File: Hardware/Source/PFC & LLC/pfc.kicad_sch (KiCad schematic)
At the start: 56 parts, among them J1 HB9500M-9.5-3P, K1 Relay 12VDC 10A, Q1 MMBT2222A, Q2 IPP60R125CP, Q3 MMBT2222A, U2 PC817X2NIPW, U3 SN74LVC1G14DBVR, U4 UCC28180D

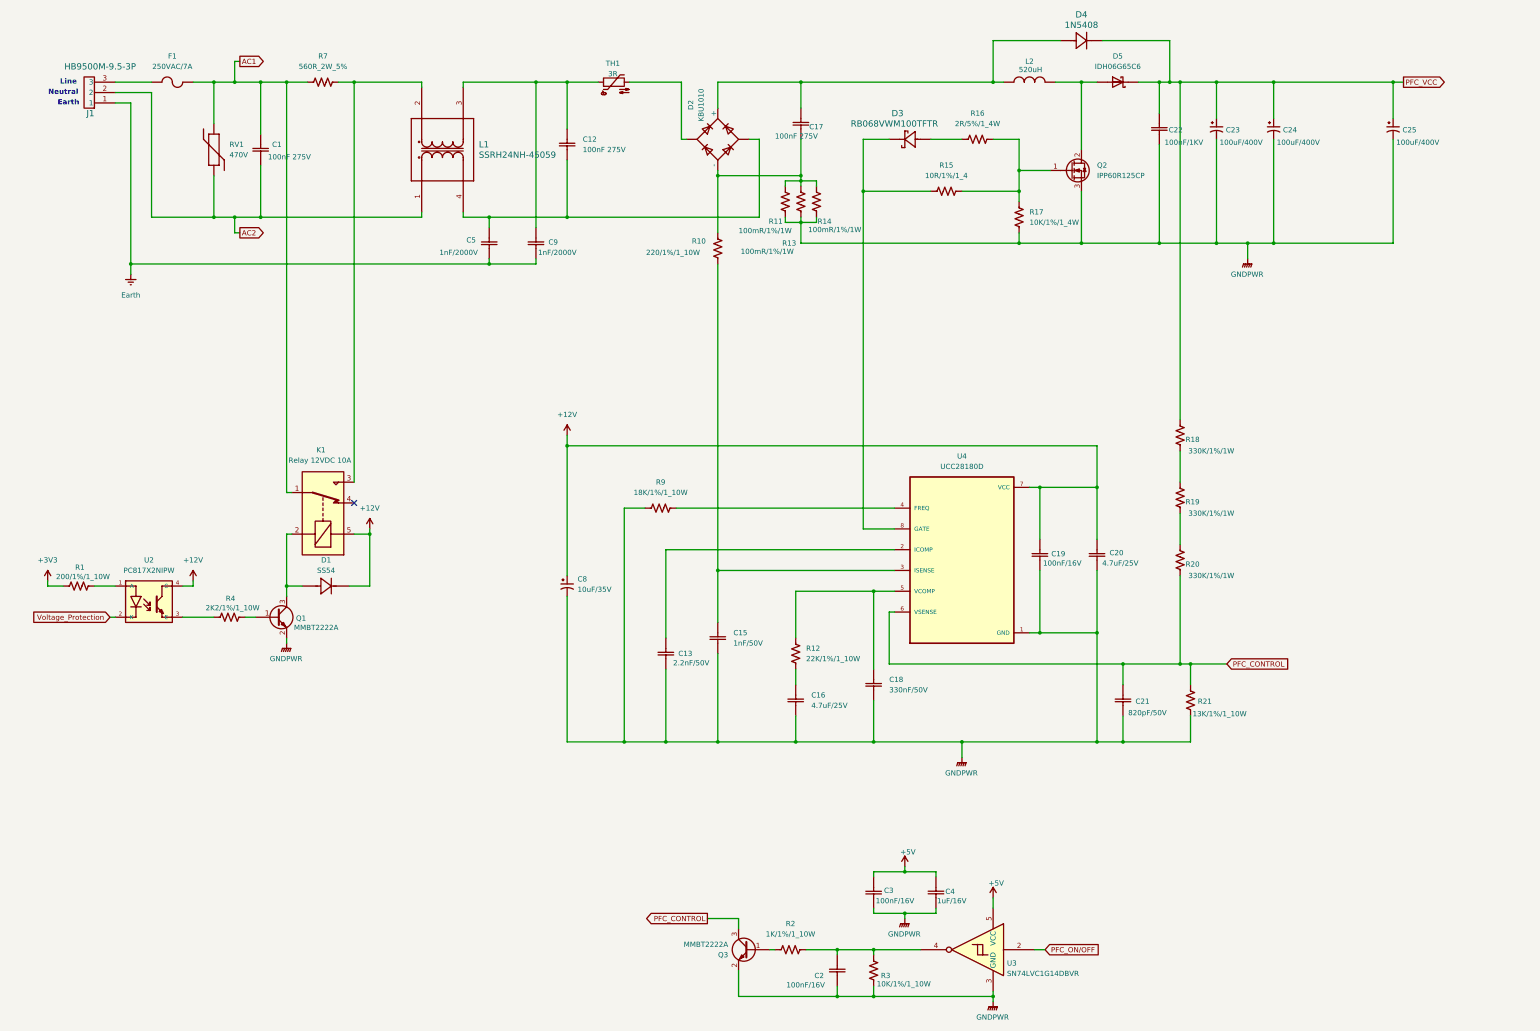
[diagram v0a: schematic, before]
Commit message: update FEEDBACK, AC
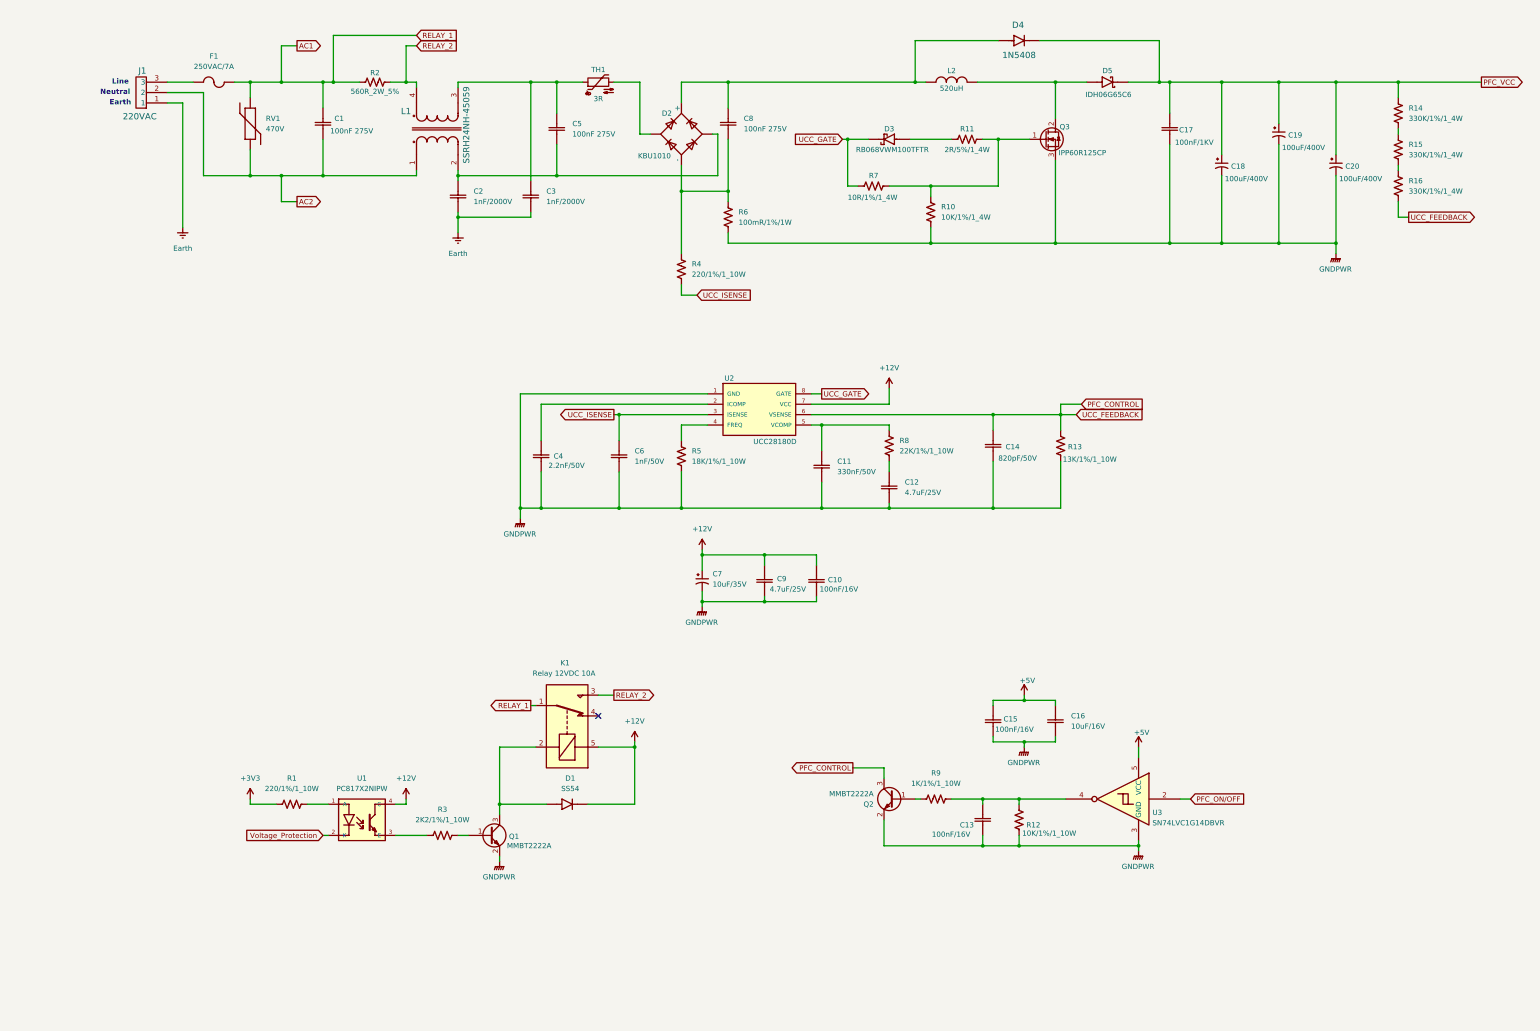
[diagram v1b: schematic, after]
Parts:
- removed C13: 2.2nF/50V, charge_battery_footprint_lib:Ceramic_Cap_0805, symbol charge_battery_sym_lib:Ceramic_Cap_SMD_2.2nF_50V
- removed C15: 1nF/50V, charge_battery_footprint_lib:Ceramic_Cap_0603, symbol charge_battery_sym_lib:Ceramic_Cap_SMD_1nF_50V
- removed C16, C20: 4.7uF/25V, charge_battery_footprint_lib:Ceramic_Cap_0603, symbol charge_battery_sym_lib:Ceramic_Cap_SMD_4.7uF_25V
- removed C17: 100nF 275V, charge_battery_footprint_lib:Candy_Cap_hole_100nF_275V, symbol charge_battery_sym_lib:Candy_Cap_hole_100nF_275V
- removed C18: 330nF/50V, charge_battery_footprint_lib:Ceramic_Cap_0603, symbol charge_battery_sym_lib:Ceramic_Cap_SMD_330nF_50V
- removed C19: 100nF/16V, charge_battery_footprint_lib:Ceramic_Cap_0603, symbol charge_battery_sym_lib:Ceramic_Cap_SMD_100nF_16V
- removed C21: 820pF/50V, charge_battery_footprint_lib:Ceramic_Cap_0805, symbol charge_battery_sym_lib:Ceramic_Cap_SMD_820pF_50V
- removed C4: 1uF/16V, charge_battery_footprint_lib:Ceramic_Cap_0603, symbol charge_battery_sym_lib:Ceramic_Cap_SMD_1uF_16V
- removed C5, C9: 1nF/2000V, charge_battery_footprint_lib:Ceramic_Cap_Hole_5mm, symbol charge_battery_sym_lib:Ceramic_Cap_Hole_1nF_2000V
- removed C8: 10uF/35V, charge_battery_footprint_lib:Tan_Cap_C, symbol charge_battery_sym_lib:Cap_Tantalum_10uF_35V
- removed L1: SSRH24NH-45059, charge_battery_footprint_lib:TPCM-1.7-5, symbol charge_battery_sym_lib:TPCM-1.7-5
- removed R1: 200/1%/1_10W, charge_battery_footprint_lib:Res_0603, symbol charge_battery_sym_lib:Res_200R_0603_1%
- removed R10: 220/1%/1_10W, charge_battery_footprint_lib:Res_0603, symbol charge_battery_sym_lib:Res_220R_0603_1%
- removed R11, R13, R14: 100mR/1%/1W, charge_battery_footprint_lib:Res_1206, symbol charge_battery_sym_lib:Res_100mR_1206_1%
- removed R12: 22K/1%/1_10W, charge_battery_footprint_lib:Res_0603, symbol charge_battery_sym_lib:Res_22K_0603_1%
- removed R18, R19, R20: 330K/1%/1W, charge_battery_footprint_lib:Res_1206, symbol charge_battery_sym_lib:Res_330K_1206_1%
- removed R21: 13K/1%/1_10W, charge_battery_footprint_lib:Res_0603, symbol charge_battery_sym_lib:Res_13K_0603_1%
- removed R4: 2K2/1%/1_10W, charge_battery_footprint_lib:Res_0603, symbol charge_battery_sym_lib:Res_2K2_0603_1%
- removed R9: 18K/1%/1_10W, charge_battery_footprint_lib:Res_0603, symbol charge_battery_sym_lib:Res_18K_0603_1%
- removed U4: UCC28180D, charge_battery_footprint_lib:SOIC-8, symbol charge_battery_sym_lib:UCC28180D
- added C10: 100nF/16V, charge_battery_footprint_lib:Ceramic_Cap_0603, symbol charge_battery_sym_lib:Ceramic_Cap_SMD_100nF_16V
- added C11: 330nF/50V, charge_battery_footprint_lib:Ceramic_Cap_0603, symbol charge_battery_sym_lib:Ceramic_Cap_SMD_330nF_50V
- added C12, C9: 4.7uF/25V, charge_battery_footprint_lib:Ceramic_Cap_0603, symbol charge_battery_sym_lib:Ceramic_Cap_SMD_4.7uF_25V
- added C14: 820pF/50V, charge_battery_footprint_lib:Ceramic_Cap_0805, symbol charge_battery_sym_lib:Ceramic_Cap_SMD_820pF_50V
- added C16: 10uF/16V, charge_battery_footprint_lib:Ceramic_Cap_0603, symbol charge_battery_sym_lib:Ceramic_Cap_SMD_10uF_16V
- added C2, C3: 1nF/2000V, charge_battery_footprint_lib:Ceramic_Cap_Hole_5mm, symbol charge_battery_sym_lib:Ceramic_Cap_Hole_1nF_2000V
- added C4: 2.2nF/50V, charge_battery_footprint_lib:Ceramic_Cap_0805, symbol charge_battery_sym_lib:Ceramic_Cap_SMD_2.2nF_50V
- added C6: 1nF/50V, charge_battery_footprint_lib:Ceramic_Cap_0603, symbol charge_battery_sym_lib:Ceramic_Cap_SMD_1nF_50V
- added C7: 10uF/35V, charge_battery_footprint_lib:Tan_Cap_C, symbol charge_battery_sym_lib:Cap_Tantalum_10uF_35V
- added C8: 100nF 275V, charge_battery_footprint_lib:Candy_Cap_hole_100nF_275V, symbol charge_battery_sym_lib:Candy_Cap_hole_100nF_275VAC
- added L1: SSRH24NH-45059, charge_battery_footprint_lib:SSRH24NH-45059, symbol charge_battery_sym_lib:SSRH24NH-45059
- added R1, R4: 220/1%/1_10W, charge_battery_footprint_lib:Res_0603, symbol charge_battery_sym_lib:Res_220R_0603_1%
- added R13: 13K/1%/1_10W, charge_battery_footprint_lib:Res_0603, symbol charge_battery_sym_lib:Res_13K_0603_1%
- added R14, R15, R16: 330K/1%/1_4W, charge_battery_footprint_lib:Res_1206, symbol charge_battery_sym_lib:Res_330K_1206_1%
- added R3: 2K2/1%/1_10W, charge_battery_footprint_lib:Res_0603, symbol charge_battery_sym_lib:Res_2K2_0603_1%
- added R5: 18K/1%/1_10W, charge_battery_footprint_lib:Res_0603, symbol charge_battery_sym_lib:Res_18K_0603_1%
- added R6: 100mR/1%/1W, charge_battery_footprint_lib:Res_1206, symbol charge_battery_sym_lib:Res_100mR_1206_1%
- added R8: 22K/1%/1_10W, charge_battery_footprint_lib:Res_0603, symbol charge_battery_sym_lib:Res_22K_0603_1%
- added U2: UCC28180D, charge_battery_footprint_lib:SOIC-8, symbol charge_battery_sym_lib:UCC28180D
- J1: value HB9500M-9.5-3P -> 220VAC
- R7: renamed from R15; value 10R/1%/1_4 -> 10R/1%/1_4W
- U1: renamed from U2; Supply name Thegioiic -> (none); Supply name  (none) -> Thegioiic
- renumbered C2 to C13, C3 to C15, C22 to C17, C23 to C18, C24 to C19, C25 to C20, C12 to C5, Q3 to Q2, Q2 to Q3, R17 to R10, R16 to R11, R3 to R12, R7 to R2, R2 to R9
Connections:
- net +12V: now also C10.2, C7.1, C9.2, U2.7 (VCC)
- net +3V3: now also R1.2
- net +5V: now also C16.2
- net AC2: now also L1.1
- net Earth: now also C2.1, C3.1
- net GNDPWR: now also C10.1, C11.1, C12.1, C14.1, C16.1, C4.1, C6.1, C7.2, C9.1, R13.1, R5.1, R6.1, U2.1 (GND)
- net PFC_CONTROL: now also C14.2, R13.2, R16.2, U2.6 (VSENSE)
- net PFC_VCC: now also R14.1
- net at D2.4 (-): now also C8.1, R4.2, R6.2
- net at U1.3 (E): now also R3.1
- net at Q1.1 (B): now also R3.2
- net at C5.1, D2.2: now also C2.2, L1.2
- net at D2.1 (+), D4.2, L2.1: now also C8.2
- net at C5.2, TH1.1: now also C3.2, L1.3
- net RELAY_2: now reaches K1.3, R2.2
- net RELAY_2: now also L1.4
- net UCC_GATE: now reaches D3.1, R7.1
- net UCC_GATE: now also U2.8 (GATE)
- net at U1.1 (A): now also R1.1
- new net: C11.2, R8.2, U2.5 (VCOMP)
- new net: C4.2, U2.2 (ICOMP)
- new net: R5.2, U2.4 (FREQ)
- new net: R15.2, R16.1
- new net: R14.2, R15.1
- new net: C12.2, R8.1
- new net UCC_ISENSE: C6.2, R4.1, U2.3 (ISENSE)
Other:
- moved on the sheet: C1, C13, C15, C17, C18, C19, C20, C5, D2, D3, D4, D5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
